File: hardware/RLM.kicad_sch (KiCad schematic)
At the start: 1 part, among them U1 ESP32-DEVKIT-V1

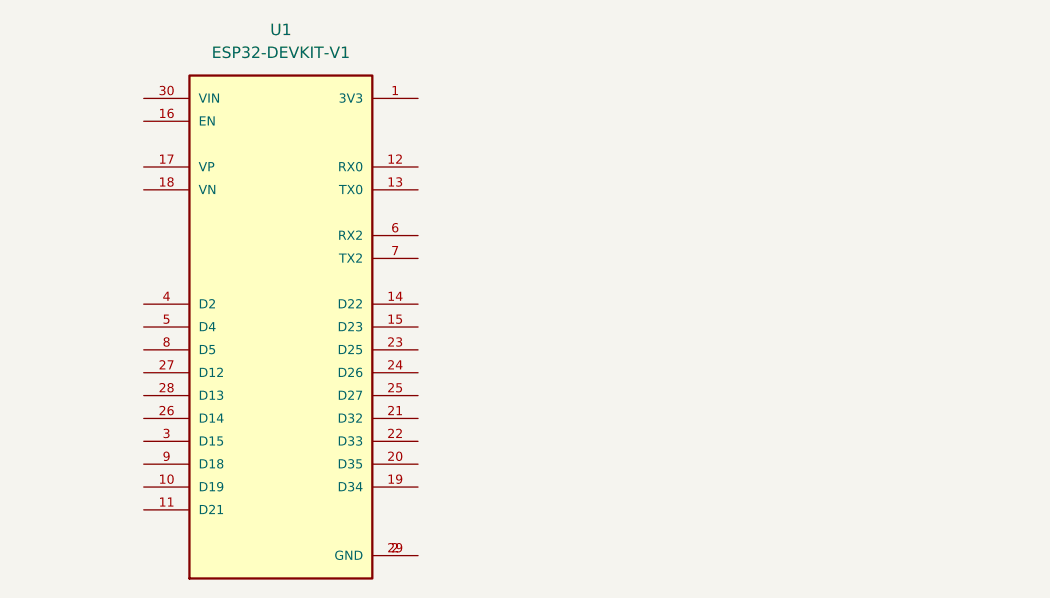
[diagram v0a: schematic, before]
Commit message: feat: add nRF module
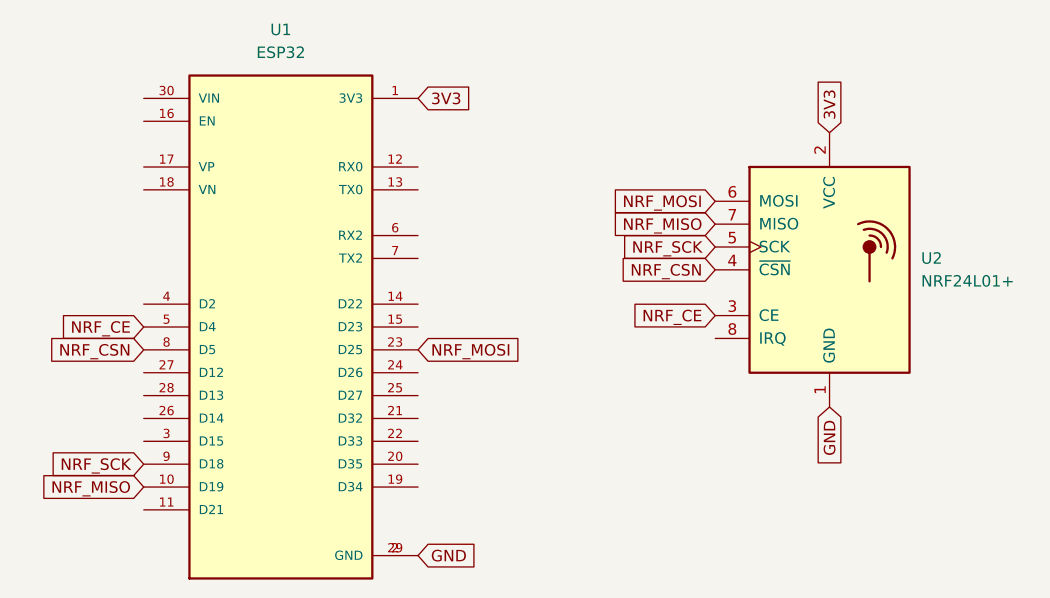
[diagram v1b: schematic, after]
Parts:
- added U2: NRF24L01+, RF_Module:nRF24L01_Breakout, symbol RF:NRF24L01_Breakout
- U1: value ESP32-DEVKIT-V1 -> ESP32; footprint ESP32-DEVKIT-V1:MODULE_ESP32_DEVKIT_V1 -> GRC:MODULE_ESP32_DEVKIT_V1
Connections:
- net 3V3: now reaches U1.1 (3V3)
- net 3V3: now also U2.2 (VCC)
- net NRF_MISO: now reaches U1.10 (D19)
- net NRF_MISO: now also U2.7 (MISO)
- net GND: now reaches U1.2 (GND), U1.29 (GND)
- net GND: now also U2.1 (GND)
- net NRF_MOSI: now reaches U1.23 (D25)
- net NRF_MOSI: now also U2.6 (MOSI)
- net NRF_CE: now reaches U1.5 (D4)
- net NRF_CE: now also U2.3 (CE)
- net NRF_CSN: now reaches U1.8 (D5)
- net NRF_CSN: now also U2.4 (~{CSN})
- net NRF_SCK: now reaches U1.9 (D18)
- net NRF_SCK: now also U2.5 (SCK)
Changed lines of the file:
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@@
 (kicad_sch (version 20230121) (generator eeschema)
   (paper "A4")
+  (global_label "NRF_MISO" (shape input) (at 125.73 128.27 180) (fields_autoplaced)
+    (effects (font (size 1.27 1.27)) (justify right))
+    (property "Intersheetrefs" "${INTERSHEET_REFS}" (at 113.4919 128.27 0)
+      (effects (font (size 1.27 1.27)) (justify right) hide)
+    )
+  )
+  (global_label "GND" (shape input) (at 201.93 119.38 270) (fields_autoplaced)
+    (effects (font (size 1.27 1.27)) (justify right))
+    (property "Intersheetrefs" "${INTERSHEET_REFS}" (at 201.93 126.2357 90)
+      (effects (font (size 1.27 1.27)) (justify right) hide)
+    )
+  )
+  (global_label "NRF_MISO" (shape input) (at 189.23 99.06 180) (fields_autoplaced)
+    (effects (font (size 1.27 1.27)) (justify right))
+    (property "Intersheetrefs" "${INTERSHEET_REFS}" (at 176.9919 99.06 0)
+      (effects (font (size 1.27 1.27)) (justify right) hide)
+    )
+  )
+  (global_label "NRF_CSN" (shape input) (at 125.73 113.03 180) (fields_autoplaced)
+    (effects (font (size 1.27 1.27)) (justify right))
+    (property "Intersheetrefs" "${INTERSHEET_REFS}" (at 114.2781 113.03 0)
+      (effects (font (size 1.27 1.27)) (justify right) hide)
+    )
+  )
+  (global_label "NRF_MOSI" (shape input) (at 156.21 113.03 0) (fields_autoplaced)
+    (effects (font (size 1.27 1.27)) (justify left))
+    (property "Intersheetrefs" "${INTERSHEET_REFS}" (at 168.4481 113.03 0)
+      (effects (font (size 1.27 1.27)) (justify left) hide)
+    )
+  )
+  (global_label "3V3" (shape input) (at 201.93 88.9 90) (fields_autoplaced)
+    (effects (font (size 1.27 1.27)) (justify left))
+    (property "Intersheetrefs" "${INTERSHEET_REFS}" (at 201.93 82.4072 90)
+      (effects (font (size 1.27 1.27)) (justify left) hide)
+    )
+  )
+  (global_label "GND" (shape input) (at 156.21 135.89 0) (fields_autoplaced)
+    (effects (font (size 1.27 1.27)) (justify left))
+    (property "Intersheetrefs" "${INTERSHEET_REFS}" (at 163.0657 135.89 0)
+      (effects (font (size 1.27 1.27)) (justify left) hide)
+    )
+  )
+  (global_label "NRF_CE" (shape input) (at 189.23 109.22 180) (fields_autoplaced)
+    (effects (font (size 1.27 1.27)) (justify right))
+    (property "Intersheetrefs" "${INTERSHEET_REFS}" (at 179.1691 109.22 0)
+      (effects (font (size 1.27 1.27)) (justify right) hide)
+    )
+  )
+  (global_label "NRF_SCK" (shape input) (at 189.23 101.6 180) (fields_autoplaced)
+    (effects (font (size 1.27 1.27)) (justify right))
+    (property "Intersheetrefs" "${INTERSHEET_REFS}" (at 177.8386 101.6 0)
+      (effects (font (size 1.27 1.27)) (justify right) hide)
+    )
+  )
+  (global_label "NRF_CSN" (shape input) (at 189.23 104.14 180) (fields_autoplaced)
+    (effects (font (size 1.27 1.27)) (justify right))
+    (property "Intersheetrefs" "${INTERSHEET_REFS}" (at 177.7781 104.14 0)
+      (effects (font (size 1.27 1.27)) (justify right) hide)
+    )
+  )
+  (global_label "NRF_SCK" (shape input) (at 125.73 125.73 180) (fields_autoplaced)
+    (effects (font (size 1.27 1.27)) (justify right))
+    (property "Intersheetrefs" "${INTERSHEET_REFS}" (at 114.3386 125.73 0)
+      (effects (font (size 1.27 1.27)) (justify right) hide)
+    )
+  )
+  (global_label "NRF_MOSI" (shape input) (at 189.23 96.52 180) (fields_autoplaced)
+    (effects (font (size 1.27 1.27)) (justify right))
+    (property "Intersheetrefs" "${INTERSHEET_REFS}" (at 176.9919 96.52 0)
+      (effects (font (size 1.27 1.27)) (justify right) hide)
+    )
+  )
+  (global_label "3V3" (shape input) (at 156.21 85.09 0) (fields_autoplaced)
+    (effects (font (size 1.27 1.27)) (justify left))
+    (property "Intersheetrefs" "${INTERSHEET_REFS}" (at 162.7028 85.09 0)
+      (effects (font (size 1.27 1.27)) (justify left) hide)
+    )
+  )
+  (global_label "NRF_CE" (shape input) (at 125.73 110.49 180) (fields_autoplaced)
+    (effects (font (size 1.27 1.27)) (justify right))
+    (property "Intersheetrefs" "${INTERSHEET_REFS}" (at 115.6691 110.49 0)
+      (effects (font (size 1.27 1.27)) (justify right) hide)
+    )
+  )
+  (symbol (lib_id "RF:NRF24L01_Breakout") (at 201.93 104.14 0) (unit 1)
+    (in_bom yes) (on_board yes) (dnp no) (fields_autoplaced)
+    (property "Reference" "U2" (at 212.09 102.87 0)
+      (effects (font (size 1.27 1.27)) (justify left))
+    )
+    (property "Value" "NRF24L01+" (at 212.09 105.41 0)
+      (effects (font (size 1.27 1.27)) (justify left))
+    )
+    (property "Footprint" "RF_Module:nRF24L01_Breakout" (at 205.74 88.9 0)
+      (effects (font (size 1.27 1.27) italic) (justify left) hide)
+    )
+    (property "Datasheet" "http://www.nordicsemi.com/eng/content/download/2730/34105/file/nRF24L01_Product_Specification_v2_0.pdf" (at 201.93 106.68 0)
+      (effects (font (size 1.27 1.27)) hide)
+    )
+    (pin "1")
+    (pin "2")
+    (pin "3")
+    (pin "4")
+    (pin "5")
+    (pin "6")
+    (pin "7")
+    (pin "8")
+    (instances
+      (project "RLM"
+        (path "/3fe8a1ac-6190-4220-82eb-f4588302947e"
+          (reference "U2") (unit 1)
+        )
+      )
+    )
+  )
   (symbol (lib_id "GRC_ESP32-DEVKIT-V1:ESP32-DEVKIT-V1") (at 140.97 110.49 0) (unit 1)
     (in_bom yes) (on_board yes) (dnp no) (fields_autoplaced)
@@
       (effects (font (size 1.27 1.27)))
     )
-    (property "Value" "ESP32-DEVKIT-V1" (at 140.97 80.01 0)
+    (property "Value" "ESP32" (at 140.97 80.01 0)
       (effects (font (size 1.27 1.27)))
     )
-    (property "Footprint" "ESP32-DEVKIT-V1:MODULE_ESP32_DEVKIT_V1" (at 140.97 110.49 0)
+    (property "Footprint" "GRC:MODULE_ESP32_DEVKIT_V1" (at 140.97 110.49 0)
       (effects (font (size 1.27 1.27)) (justify bottom) hide)
     )
